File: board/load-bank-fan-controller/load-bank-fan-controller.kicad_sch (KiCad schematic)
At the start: 42 parts, among them J1 UART, J10 Conn Relay, J11 Conn Temp, J12 Conn Temp, J13 Conn Temp, J2 FAN1, J3 FAN2, J4 FAN3, J5 FAN4, J6 Conn 12V, J7 SJ-3523-SMT-TR, J8 SJ-3523-SMT-TR, J9 SJ-3523-SMT-TR, Q1 IRF540N, SW1 SW_Push, U1 ATmega328P-A, U2 AMS1117-5.0, Y1 Crystal

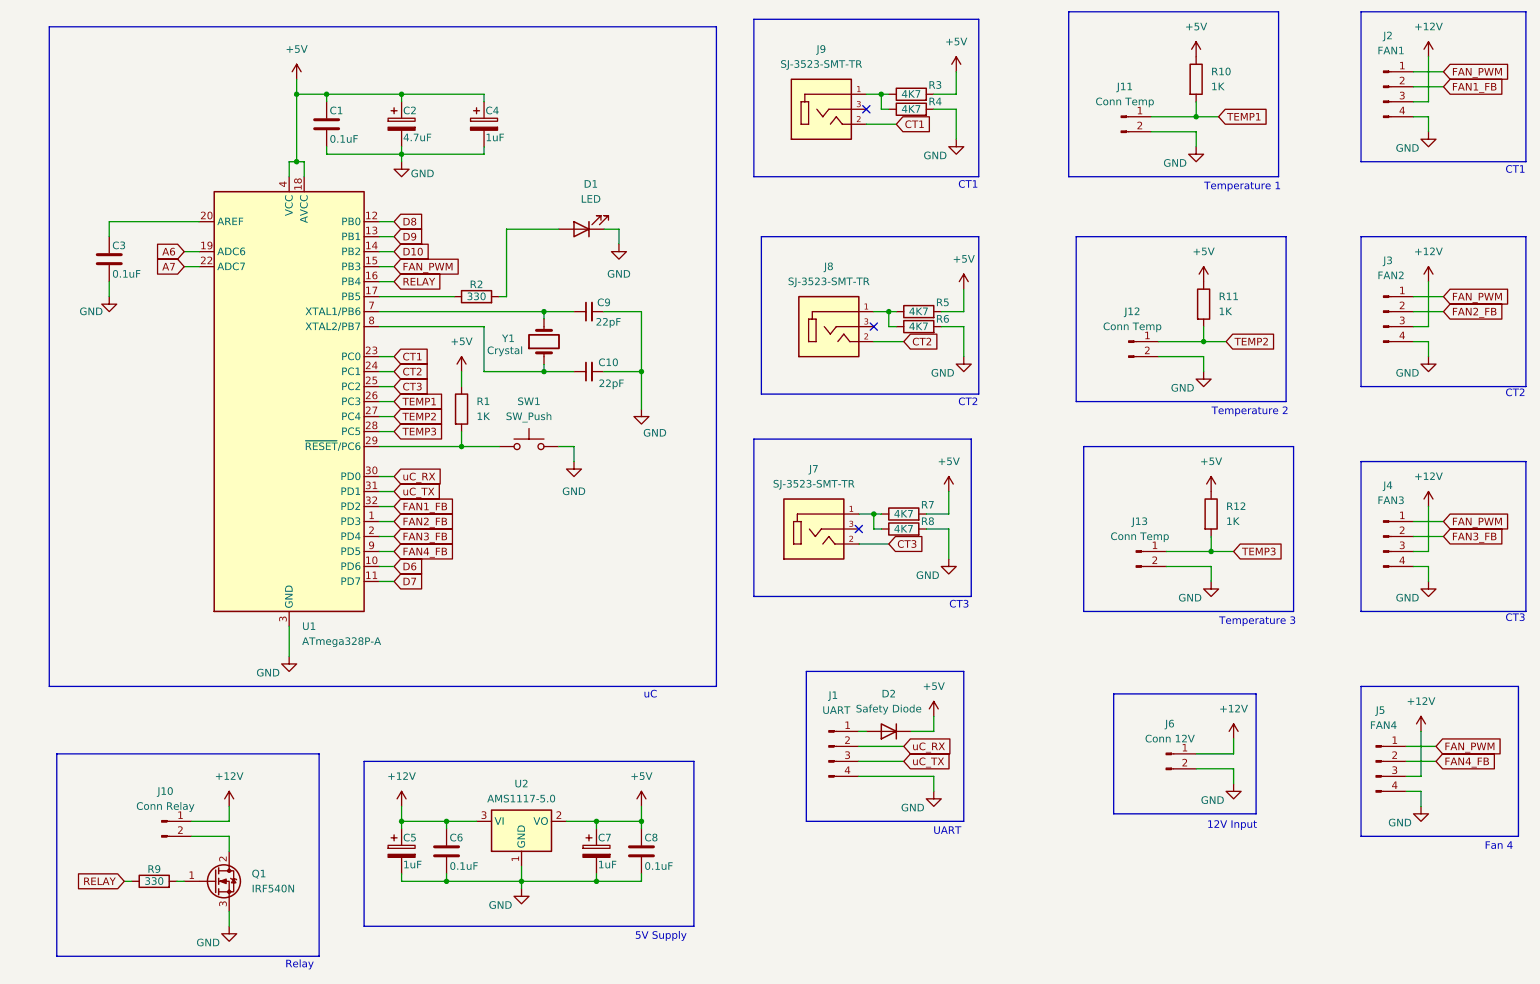
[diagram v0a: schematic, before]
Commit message: finish board routing
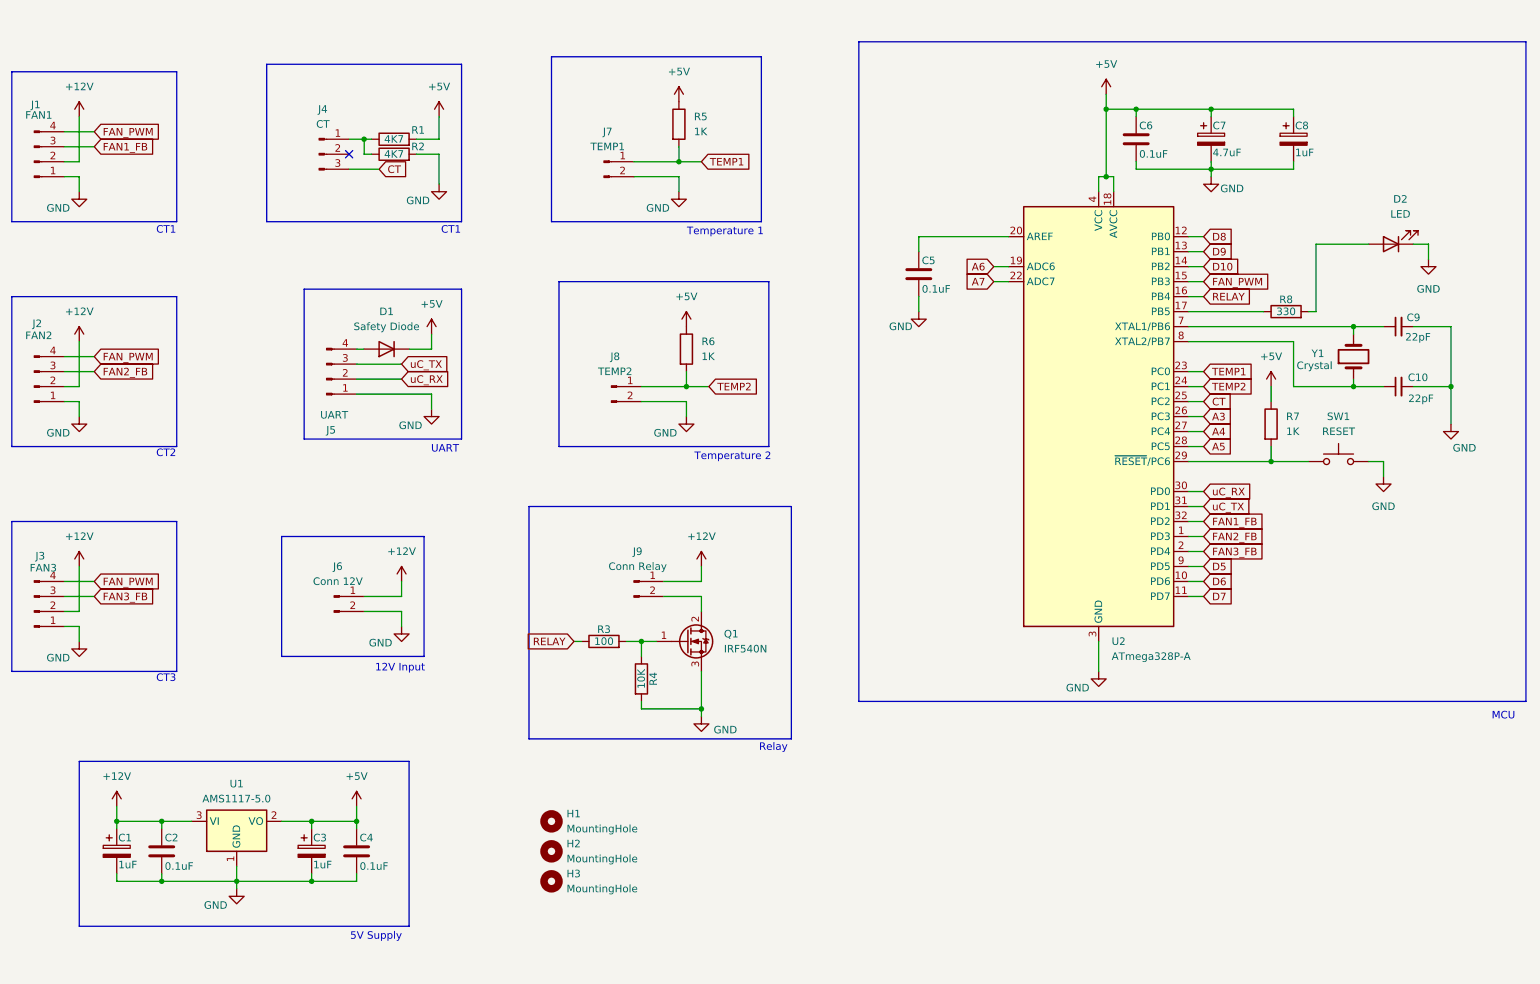
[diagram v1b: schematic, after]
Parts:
- removed J13: Conn Temp, Connector_Molex:Molex_KK-254_AE-6410-02A_1x02_P2.54mm_Vertical, symbol Connector:Conn_01x02_Pin
- removed J5: FAN4, Connector:FanPinHeader_1x04_P2.54mm_Vertical, symbol Connector:Conn_01x04_Pin
- removed J7, J8, J9: SJ-3523-SMT-TR, SJ-3523-SMT-TR:CUI_SJ-3523-SMT-TR, symbol SJ-3523-SMT-TR:SJ-3523-SMT-TR
- removed R12: 1K, Resistor_SMD:R_0603_1608Metric_Pad0.98x0.95mm_HandSolder, symbol Device:R
- removed R5, R6, R7, R8: 4K7, Resistor_SMD:R_0603_1608Metric_Pad0.98x0.95mm_HandSolder, symbol Device:R
- added H1, H2, H3: MountingHole, MountingHole:MountingHole_3.2mm_M3, symbol Mechanical:MountingHole
- added J4: CT, Connector_JST:JST_XH_B3B-XH-A_1x03_P2.50mm_Vertical, symbol Connector:Conn_01x03_Pin
- added R4: 10K, Resistor_SMD:R_0603_1608Metric_Pad0.98x0.95mm_HandSolder, symbol Device:R
- J1: renamed from J2; footprint Connector:FanPinHeader_1x04_P2.54mm_Vertical -> Connector_Molex:Molex_KK-254_AE-6410-04A_1x04_P2.54mm_Vertical
- J2: renamed from J3; footprint Connector:FanPinHeader_1x04_P2.54mm_Vertical -> Connector_Molex:Molex_KK-254_AE-6410-04A_1x04_P2.54mm_Vertical
- J3: renamed from J4; footprint Connector:FanPinHeader_1x04_P2.54mm_Vertical -> Connector_Molex:Molex_KK-254_AE-6410-04A_1x04_P2.54mm_Vertical
- J5: renamed from J1; footprint Connector_Molex:Molex_KK-254_AE-6410-04A_1x04_P2.54mm_Vertical -> Connector_JST:JST_XH_B4B-XH-A_1x04_P2.50mm_Vertical
- J7: renamed from J11; value Conn Temp -> TEMP1; footprint Connector_Molex:Molex_KK-254_AE-6410-02A_1x02_P2.54mm_Vertical -> Connector_JST:JST_XH_B2B-XH-A_1x02_P2.50mm_Vertical
- J8: renamed from J12; value Conn Temp -> TEMP2; footprint Connector_Molex:Molex_KK-254_AE-6410-02A_1x02_P2.54mm_Vertical -> Connector_JST:JST_XH_B2B-XH-A_1x02_P2.50mm_Vertical
- R3: renamed from R9; value 330 -> 100; LCSC PN C105881 -> C105588; Mfg PN RC0603FR-07330RL -> RC0603FR-07100RL
- SW1: value SW_Push -> RESET
- renumbered C5 to C1, C6 to C2, C7 to C3, C8 to C4, C3 to C5, C1 to C6, C2 to C7, C4 to C8, D2 to D1, D1 to D2, J10 to J9, R3 to R1, R4 to R2, R10 to R5, R11 to R6, R1 to R7, R2 to R8, U2 to U1, U1 to U2
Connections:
- net CT1 is gone; now on net TEMP1: U2.23 (PC0)
- net CT2 is gone; now on net TEMP2: U2.24 (PC1)
- net +12V: now also J1.2 (Pin_2), J2.2 (Pin_2), J3.2 (Pin_2); no longer J1.3 (Pin_3), J2.3 (Pin_3), J3.3 (Pin_3)
- net FAN1_FB: now also J1.3 (Pin_3); no longer J1.2 (Pin_2)
- net FAN2_FB: now also J2.3 (Pin_3); no longer J2.2 (Pin_2)
- net FAN3_FB: now also J3.3 (Pin_3); no longer J3.2 (Pin_2)
- net FAN_PWM: now also J1.4 (Pin_4), J2.4 (Pin_4), J3.4 (Pin_4); no longer J1.1 (Pin_1), J2.1 (Pin_1), J3.1 (Pin_1)
- net GND: now also J1.1 (Pin_1), J2.1 (Pin_1), J3.1 (Pin_1), J5.1 (Pin_1), R4.2; no longer J1.4 (Pin_4), J2.4 (Pin_4), J3.4 (Pin_4), J5.4 (Pin_4)
- net TEMP1: no longer U2.26 (PC3)
- net TEMP2: no longer U2.27 (PC4)
- net at D1.2 (A): now also J5.4 (Pin_4); no longer J5.1 (Pin_1)
- net at Q1.1 (G), R3.2: now also R4.1
- net at R1.1, R2.1: now also J4.1 (Pin_1)
- net CT3 renamed CT
- net CT: now also J4.3 (Pin_3)
- net FAN4_FB renamed D5
- net TEMP3 renamed A5
- new net A3: U2.26 (PC3)
- new net A4: U2.27 (PC4)
- no-connect marks 3 -> 1
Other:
- note added: "MCU"
- note removed: "Fan 4"
- note removed: "Temperature 3"
- note removed: "uC"
- moved on the sheet: C1, C10, C2, C3, C4, C5, C6, C7, C8, C9, D1, D2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
